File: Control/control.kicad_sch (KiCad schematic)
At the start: 9 parts, among them J2-J4 Conn_01x10, J3-J1 Conn_01x10, U1 TLV2372

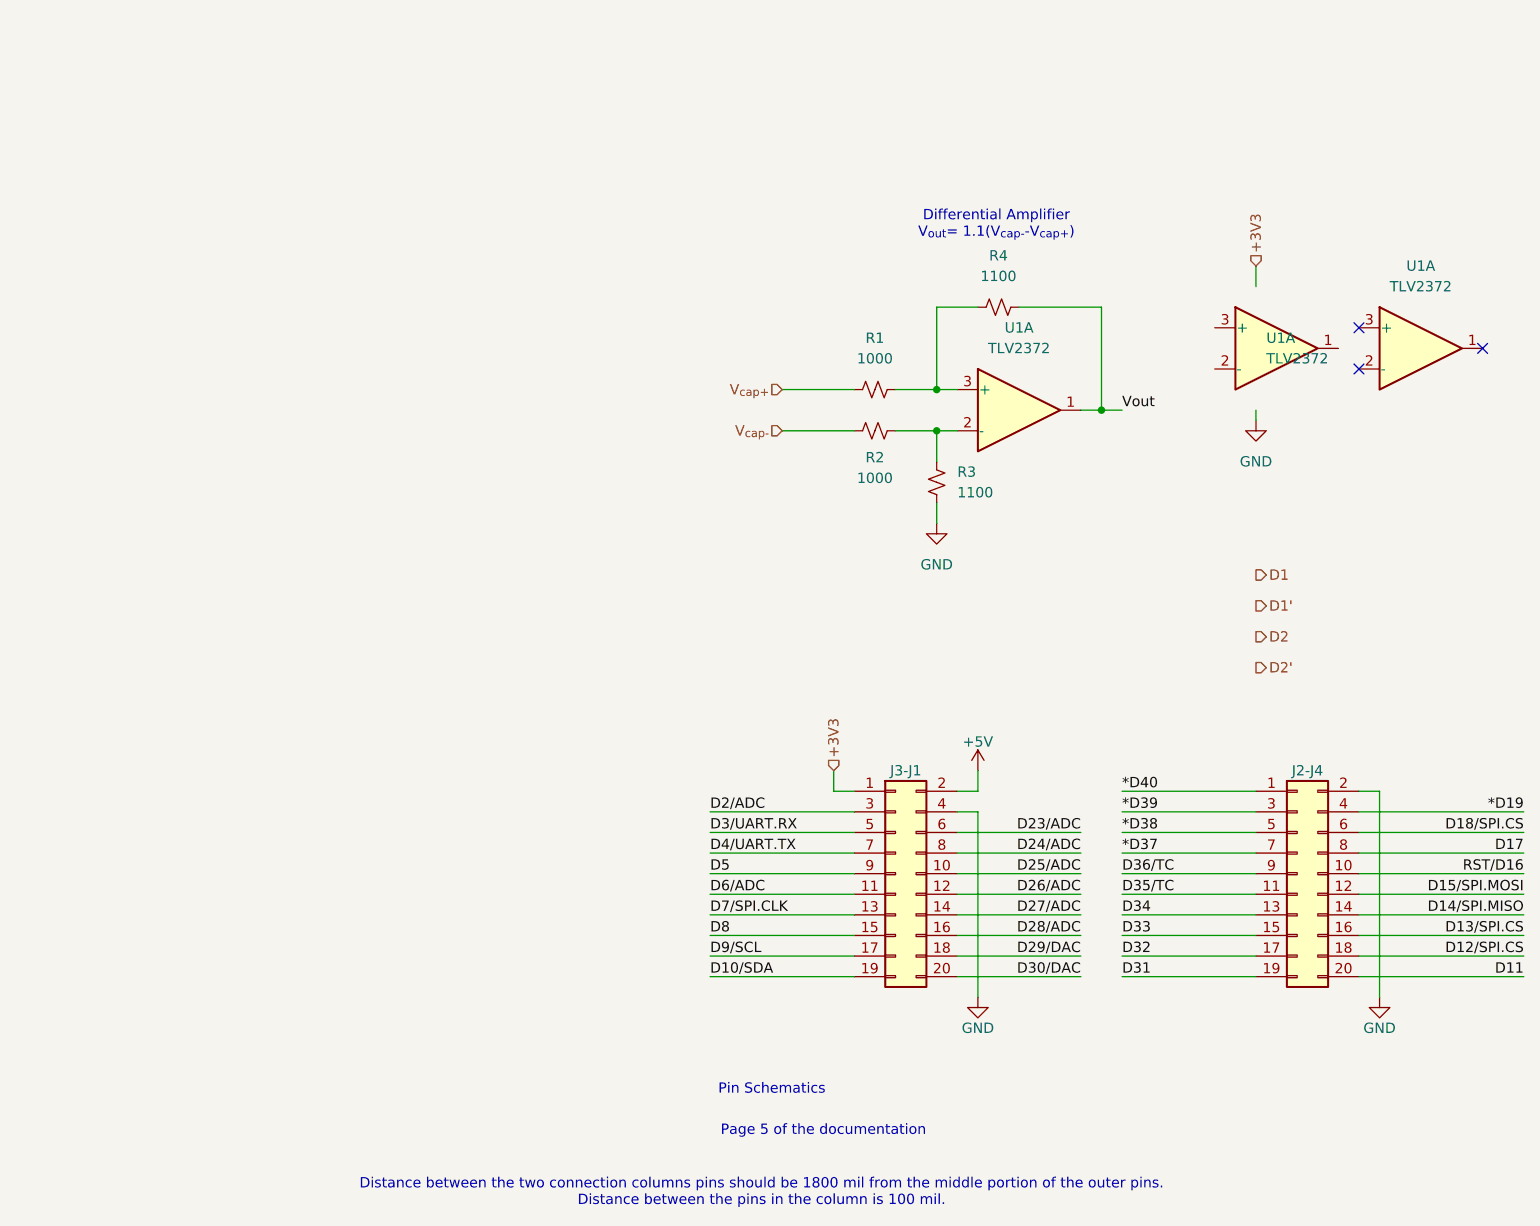
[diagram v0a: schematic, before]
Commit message: began layout
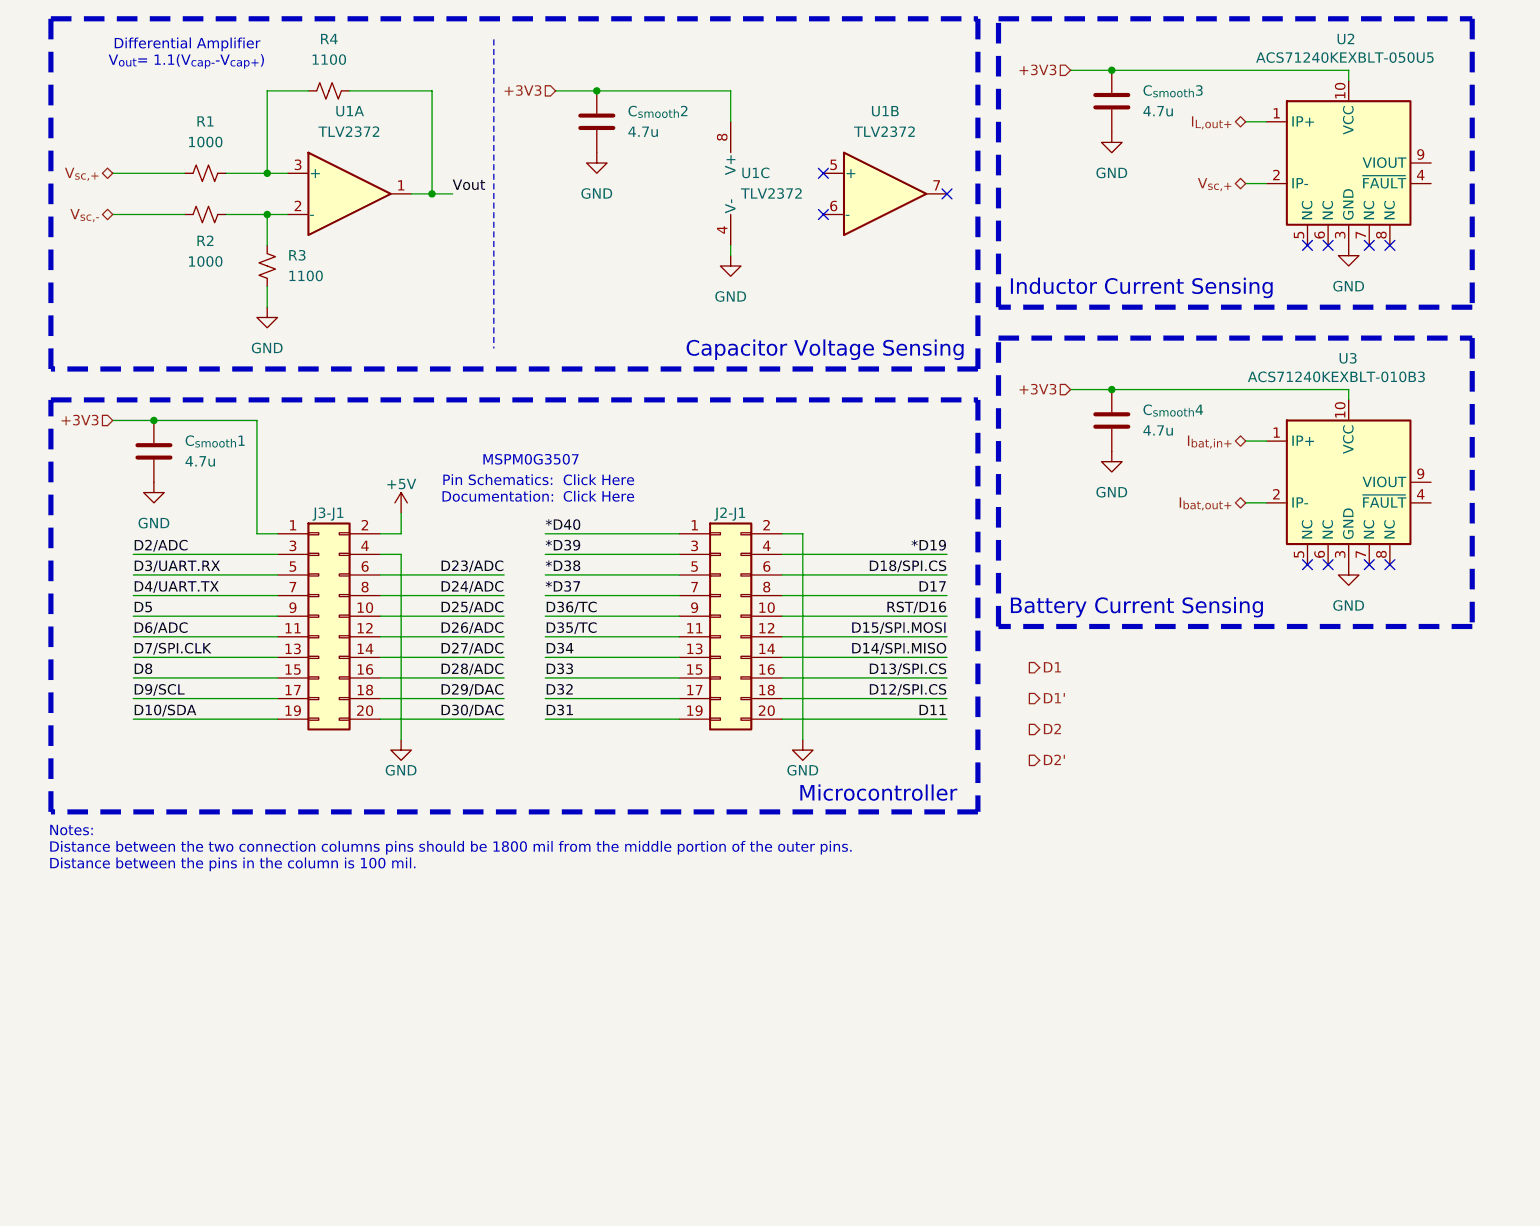
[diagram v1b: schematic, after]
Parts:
- added C_{smooth}1, C_{smooth}2, C_{smooth}3, C_{smooth}4: 4.7u, Capacitor_SMD:C_0805_2012Metric_Pad1.18x1.45mm_HandSolder, symbol Device:C
- added U2: ACS71240KEXBLT-050U5, Sensor_Current:Allegro_QFN-12-10-1EP_3x3mm_P0.5mm, symbol Sensor_Current:ACS711xEXLT-31AB
- added U3: ACS71240KEXBLT-010B3, Sensor_Current:Allegro_QFN-12-10-1EP_3x3mm_P0.5mm, symbol Sensor_Current:ACS711xEXLT-15AB
- renumbered J2-J4 to J2-J1
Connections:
- net +3V3: now also U1.8 (V+), C_{smooth}1.1, C_{smooth}2.1, C_{smooth}3.1, C_{smooth}4.1, U2.10 (VCC), U3.10 (VCC)
- net GND: now also U1.4 (V-), C_{smooth}1.2, C_{smooth}2.2, C_{smooth}3.2, C_{smooth}4.2, U2.3 (GND), U3.3 (GND)
- net V_{cap+} renamed V_{sc,+}
- net V_{sc,+}: now also U2.2 (IP-)
- net V_{cap-} renamed V_{sc,-}
- new net I_{L,out+}: U2.1 (IP+)
- new net I_{bat,in+}: U3.1 (IP+)
- new net I_{bat,out+}: U3.2 (IP-)
- no-connect marks 3 -> 11
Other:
- note added: "Battery Current Sensing"
- note added: "Capacitor Voltage Sensing"
- note added: "Click Here"
- note added: "Inductor Current Sensing"
- note added: "MSPM0G3507"
- note added: "Microcontroller"
- note added: "Notes: Distance between the two connection columns pins should be 1800 mil from the middle portion of the outer pins. Distance between the pins in the column is 100 mil."
- note added: "Pin Schematics: Documentation:"
- note removed: "Distance between the two connection columns pins should be 1800 mil from the middle portion of the outer pins. Distance between the pins in the column is 100 mil."
- note removed: "Page 5 of the documentation"
- note removed: "Pin Schematics"
- moved on the sheet: J2-J1, J3-J1, R1, R2, R3, R4, U1A, U1B
